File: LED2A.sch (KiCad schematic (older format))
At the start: 16 parts

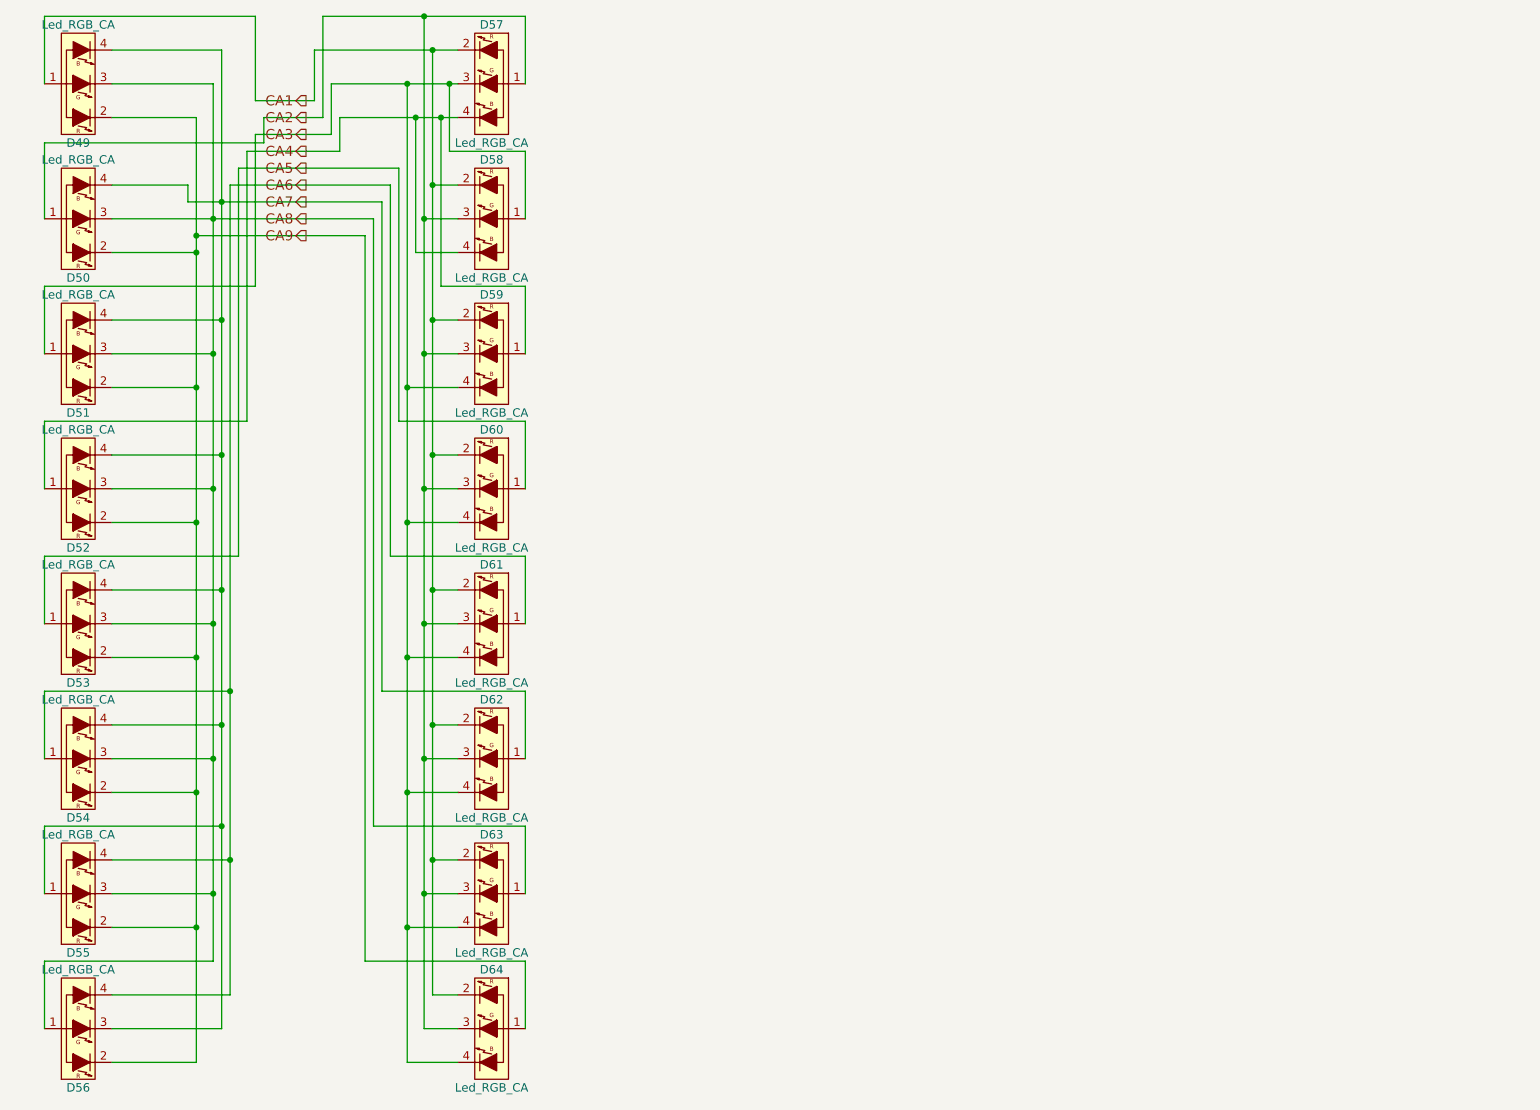
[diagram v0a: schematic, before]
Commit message: Clean up LED-Schematics
Luckily I didn't make any mistakes in the first run.
(Unless I made the same Mistake twice)
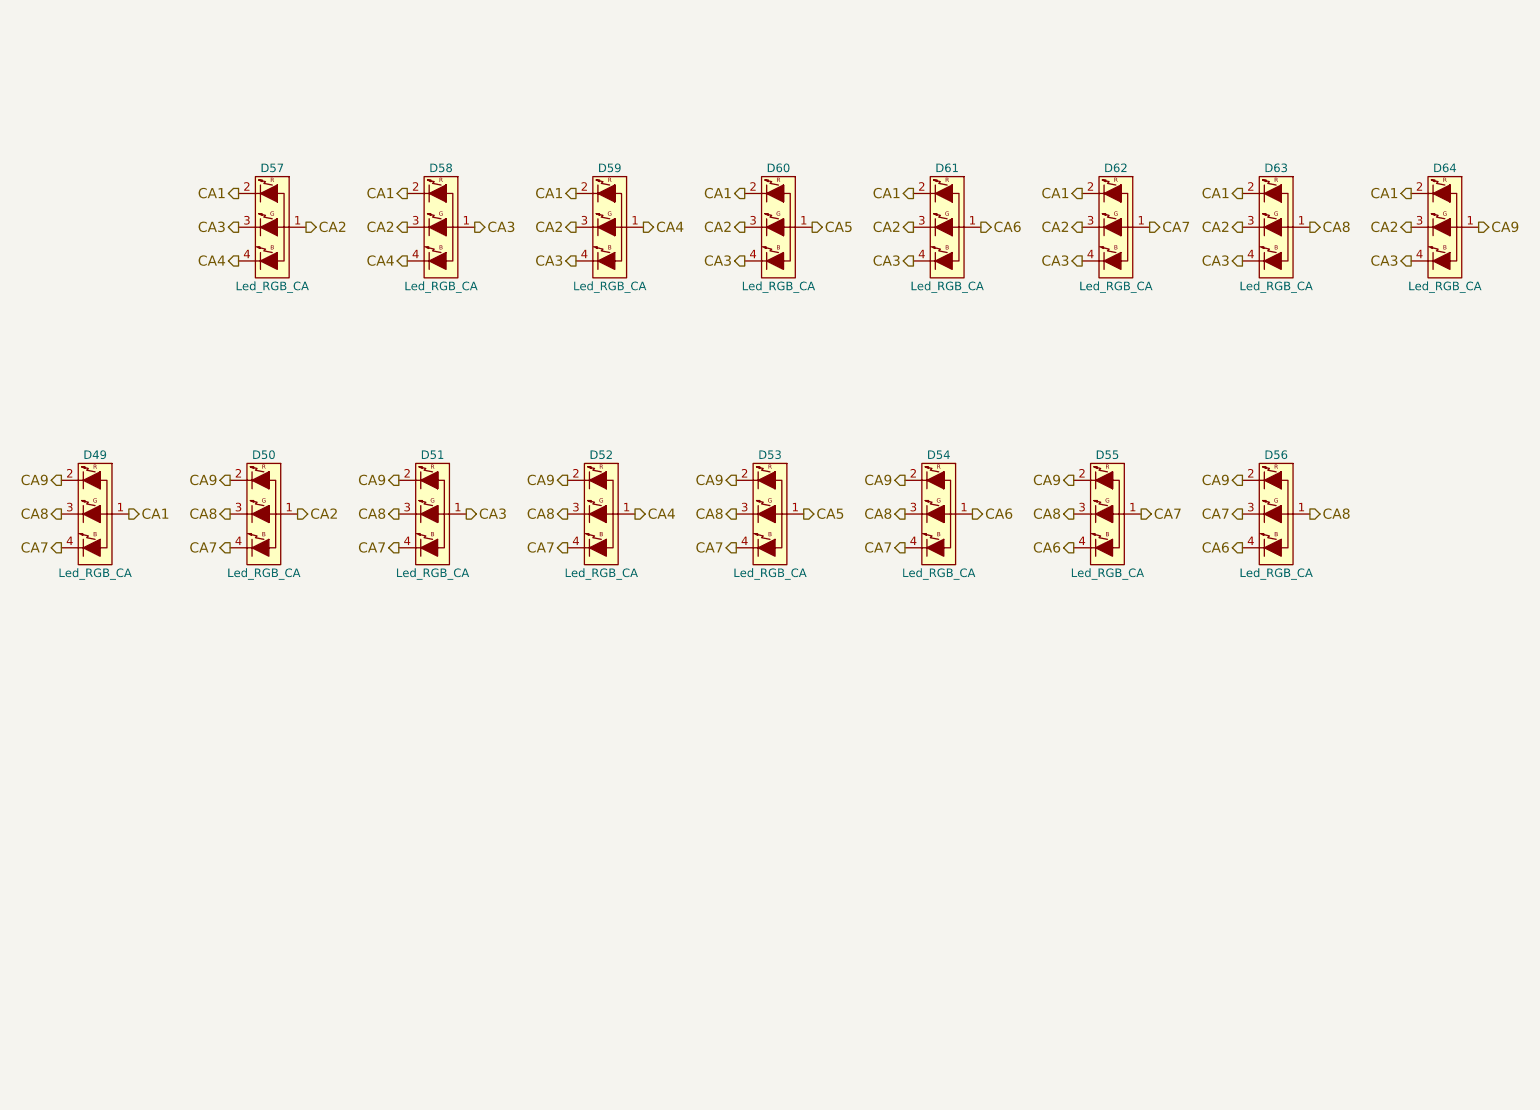
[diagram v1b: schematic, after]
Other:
- moved on the sheet: D49, D50, D51, D52, D53, D54, D55, D56, D57, D58, D59, D60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
